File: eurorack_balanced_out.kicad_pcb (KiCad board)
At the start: 2 copper layers, 60 x 35 mm, 31 parts, among them J1 Conn_01x02, J2 Conn_01x02, J3 Conn_02x05_Odd_Even, J4 AudioJack3, J5 AudioJack3, U1 THAT1646W16, U2 THAT1646W16

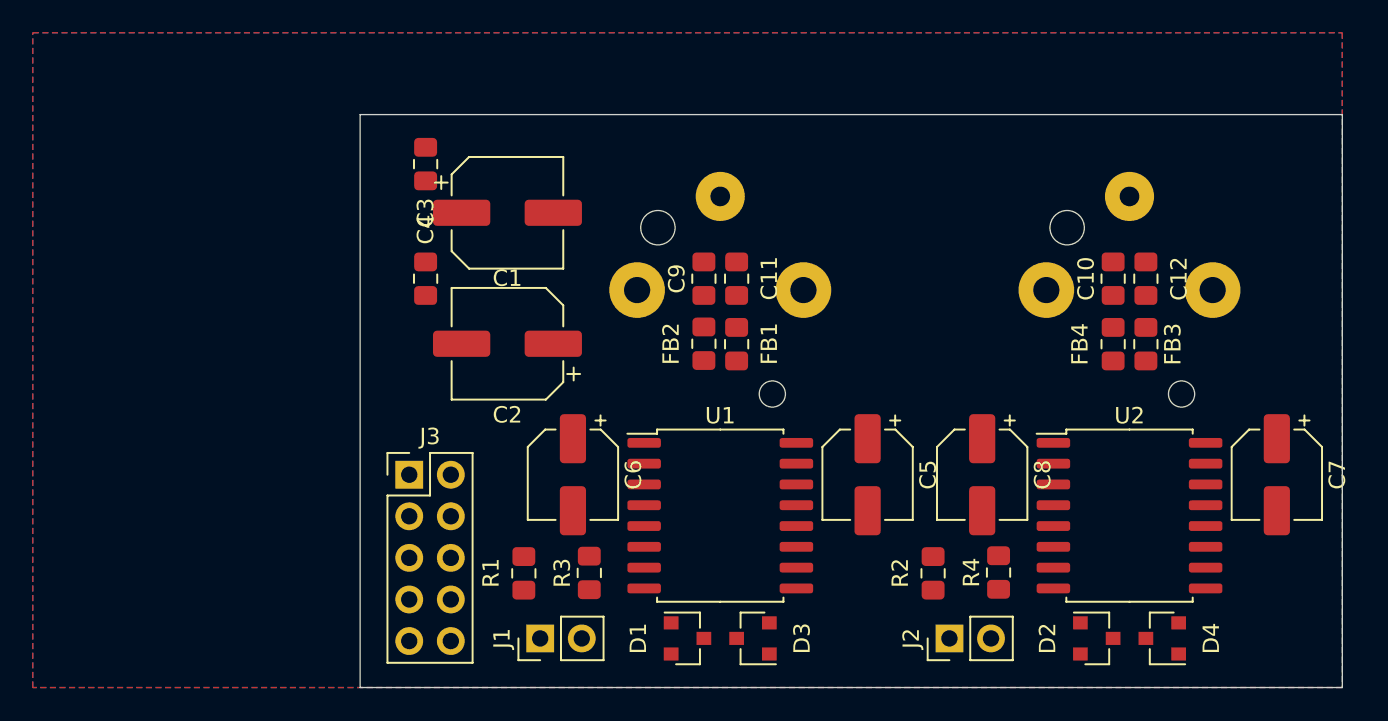
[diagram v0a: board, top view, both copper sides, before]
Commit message: route signals and some power
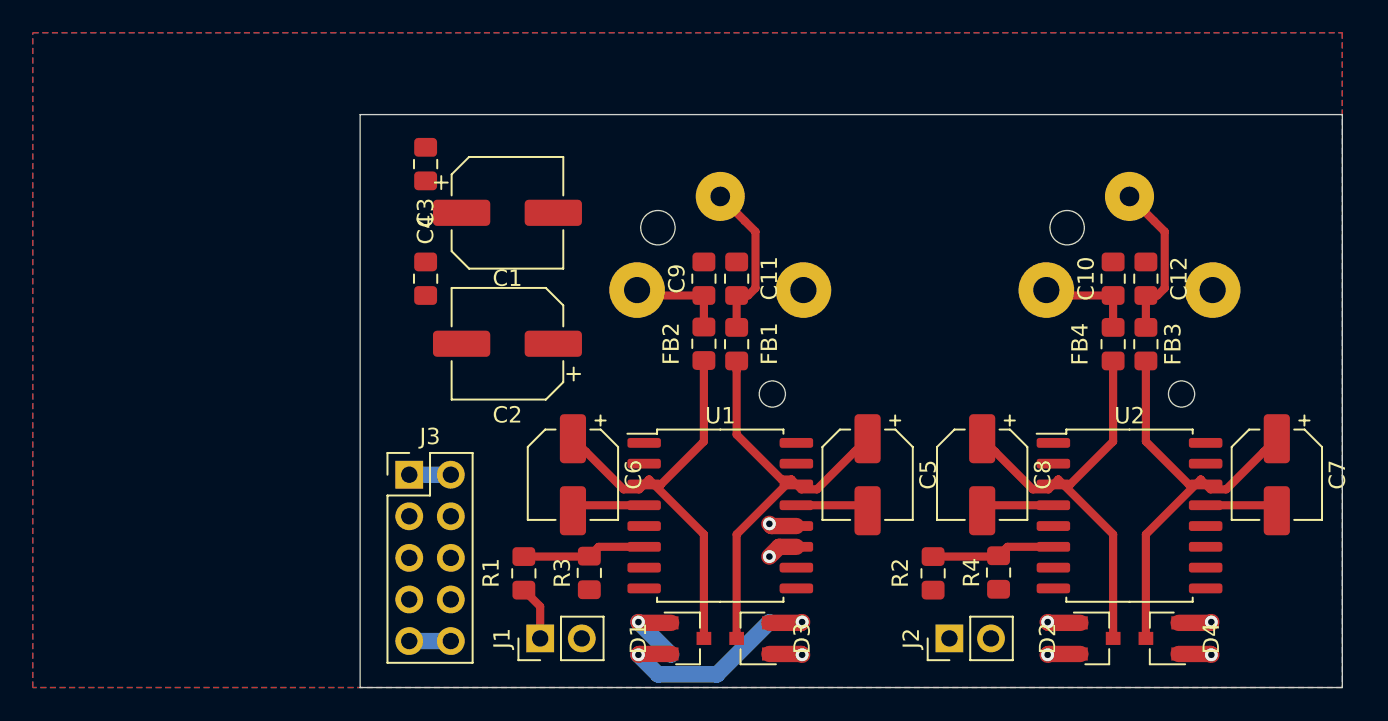
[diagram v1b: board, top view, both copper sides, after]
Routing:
- net Net-(C6-Pad1): track 0.00 -> 27.0 mm
- net Net-(C8-Pad1): track 0.00 -> 26.9 mm
- net Net-(C7-Pad1): track 0.00 -> 26.9 mm
- net Net-(C5-Pad1): track 0.00 -> 26.3 mm
- net Vcc: track 0.00 -> 22.2 mm, vias 0 -> 5
- net Vee: track 0.00 -> 15.3 mm, vias 0 -> 5
- net Net-(C12-Pad1): track 0.00 -> 9.78 mm
- net Net-(C11-Pad1): track 0.00 -> 9.78 mm
- net Net-(R2-Pad1): track 0.00 -> 7.60 mm
- net Net-(R1-Pad1): track 0.00 -> 7.60 mm
- net Net-(C10-Pad1): track 0.00 -> 6.17 mm
- net Net-(C9-Pad1): track 0.00 -> 6.14 mm
- net Net-(C8-Pad2): track 0.00 -> 4.49 mm
- net Net-(C7-Pad2): track 0.00 -> 4.49 mm
- net Net-(C6-Pad2): track 0.00 -> 4.49 mm
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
